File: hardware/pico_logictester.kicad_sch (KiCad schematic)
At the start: 29 parts, among them J1 LOGIC_INPUT, J2 GPIO_5_28, J3 AKKU, J4 STEP_UP_IN, J5 5V VERSORGUNG, J6 TFT Display, Q1 AO3401A, Q2 BC547, SW1 SW_Push, U1 74HC245, U2 74HC245

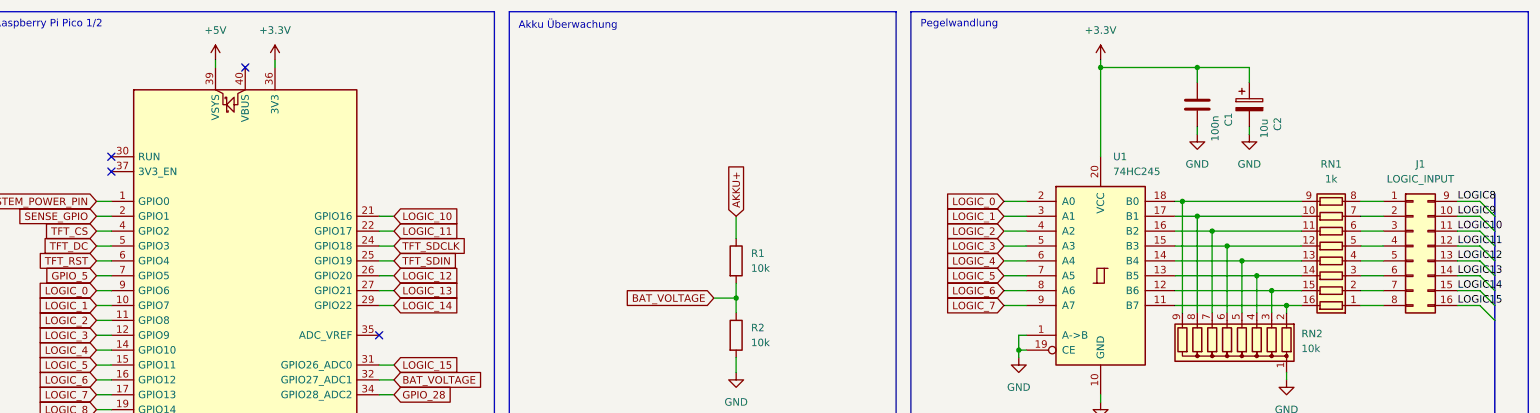
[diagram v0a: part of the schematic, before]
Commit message: Autorouting im Livestream. noch 6 offene Verbindungen!
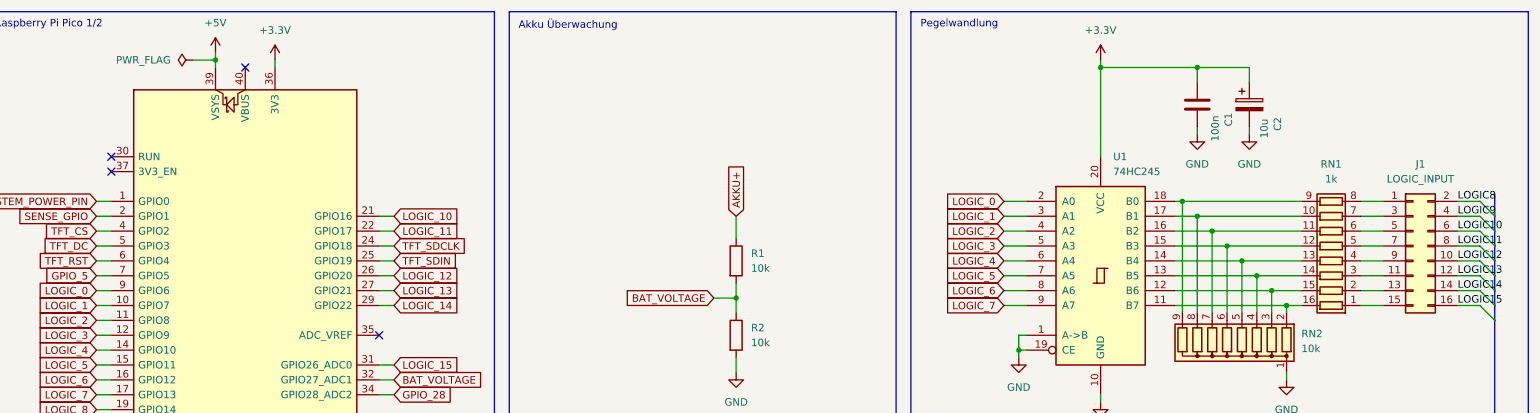
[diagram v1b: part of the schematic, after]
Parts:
- removed J1: LOGIC_INPUT, connector_tk:PinHeader_2x08_P2.54mm_Horizontal_cw, symbol Connector_Generic:Conn_02x08_Top_Bottom
- added J1: LOGIC_INPUT, Connector_IDC:IDC-Header_2x08_P2.54mm_Horizontal, symbol Connector_Generic:Conn_02x08_Odd_Even
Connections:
- net LOGIC10: now also J1.6 (Pin_6)
- net LOGIC11: now also J1.8 (Pin_8)
- net LOGIC12: now also J1.10 (Pin_10)
- net LOGIC13: now also J1.12 (Pin_12)
- net LOGIC14: now also J1.14 (Pin_14)
- net LOGIC15: now also J1.16 (Pin_16)
- net LOGIC8: now also J1.2 (Pin_2)
- net LOGIC9: now also J1.4 (Pin_4)
- net at RN1.8 (R8.1): now also J1.1 (Pin_1)
- net at RN1.7 (R7.1): now also J1.3 (Pin_3)
- net at RN1.6 (R6.1): now also J1.5 (Pin_5)
- net at RN1.5 (R5.1): now also J1.7 (Pin_7)
- net at RN1.4 (R4.1): now also J1.9 (Pin_9)
- net at RN1.3 (R3.1): now also J1.11 (Pin_11)
- net at RN1.2 (R2.1): now also J1.13 (Pin_13)
- net at RN1.1 (R1.1): now also J1.15 (Pin_15)
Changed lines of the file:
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@@
 	)
 	(junction
+		(at 58.42 22.86)
+		(diameter 0)
+		(color 0 0 0 0)
+	)
+	(junction
 		(at 226.06 99.06)
 		(diameter 0)
@@
 	(wire
 		(pts
-			(xy 58.42 22.86) (xy 58.42 24.13)
+			(xy 58.42 21.59) (xy 58.42 22.86)
 		)
 		(stroke
@@
 	(wire
 		(pts
+			(xy 58.42 22.86) (xy 58.42 24.13)
+		)
+		(stroke
+			(width 0)
+			(type default)
+		)
+	)
+	(wire
+		(pts
 			(xy 86.36 52.07) (xy 88.9 52.07)
 		)
@@
 	(wire
 		(pts
+			(xy 54.61 22.86) (xy 58.42 22.86)
+		)
+		(stroke
+			(width 0)
+			(type default)
+		)
+	)
+	(wire
+		(pts
 			(xy 195.58 72.39) (xy 195.58 73.66)
 		)
@@
 	)
 	(symbol
-		(lib_id "Connector_Generic:Conn_02x08_Top_Bottom")
-		(at 262.89 54.61 0)
-		(unit 1)
-		(exclude_from_sim no)
-		(in_bom yes)
-		(on_board yes)
-		(dnp no)
-		(fields_autoplaced yes)
-		(property "Reference" "J1"
-			(at 264.16 40.64 0)
-			(effects
-				(font
-					(size 1.27 1.27)
-				)
-			)
-		)
-		(property "Value" "LOGIC_INPUT"
-			(at 264.16 43.18 0)
-			(effects
-				(font
-					(size 1.27 1.27)
-				)
-			)
-		)
-		(property "Footprint" "connector_tk:PinHeader_2x08_P2.54mm_Horizontal_cw"
-			(at 262.89 54.61 0)
-			(effects
-				(font
-					(size 1.27 1.27)
-				)
-				(hide yes)
-			)
-		)
-		(property "Datasheet" "~"
-			(at 262.89 54.61 0)
-			(effects
-				(font
-					(size 1.27 1.27)
-				)
-				(hide yes)
-			)
-		)
-		(property "Description" "Generic connector, double row, 02x08, top/bottom pin numbering scheme (row 1: 1...pins_per_row, row2: pins_per_row+1 ... num_pins), script generated (kicad-library-utils/schlib/autogen/connector/)"
-			(at 262.89 54.61 0)
-			(effects
-				(font
-					(size 1.27 1.27)
-				)
-				(hide yes)
-			)
-		)
-		(pin "6"
-		)
-		(pin "10"
-		)
-		(pin "16"
-		)
-		(pin "13"
-		)
-		(pin "3"
-		)
-		(pin "2"
-		)
-		(pin "11"
-		)
-		(pin "4"
-		)
-		(pin "7"
-		)
-		(pin "12"
-		)
-		(pin "9"
-		)
-		(pin "5"
-		)
-		(pin "8"
-		)
-		(pin "15"
-		)
-		(pin "1"
-		)
-		(pin "14"
-		)
-		(instances
-			(project ""
-				(path "/ab4c5817-8853-4523-896c-e7a16e8d82cb"
-					(reference "J1")
-					(unit 1)
-				)
-			)
-		)
-	)
-	(symbol
 		(lib_id "Connector_Generic:Conn_01x08")
 		(at 46.99 166.37 0)
@@
 	(symbol
 		(lib_id "power:+5V")
-		(at 58.42 22.86 0)
+		(at 58.42 21.59 0)
 		(unit 1)
 		(exclude_from_sim no)
@@
 		(fields_autoplaced yes)
 		(property "Reference" "#PWR03"
-			(at 58.42 26.67 0)
+			(at 58.42 25.4 0)
 			(effects
 				(font
@@
 		)
 		(property "Value" "+5V"
-			(at 58.42 17.78 0)
+			(at 58.42 16.51 0)
 			(effects
 				(font
@@
 		)
 		(property "Footprint" ""
-			(at 58.42 22.86 0)
+			(at 58.42 21.59 0)
 			(effects
 				(font
@@
 		)
 		(property "Datasheet" ""
-			(at 58.42 22.86 0)
+			(at 58.42 21.59 0)
 			(effects
 				(font
@@
 		)
 		(property "Description" "Power symbol creates a global label with name \"+5V\""
-			(at 58.42 22.86 0)
+			(at 58.42 21.59 0)
 			(effects
 				(font
@@
 	)
 	(symbol
+		(lib_id "power:PWR_FLAG")
+		(at 54.61 22.86 90)
+		(unit 1)
+		(exclude_from_sim no)
+		(in_bom yes)
+		(on_board yes)
+		(dnp no)
+		(fields_autoplaced yes)
+		(property "Reference" "#FLG01"
+			(at 52.705 22.86 0)
+			(effects
+				(font
+					(size 1.27 1.27)
+				)
+				(hide yes)
+			)
+		)
+		(property "Value" "PWR_FLAG"
+			(at 50.8 22.8599 90)
+			(effects
+				(font
+					(size 1.27 1.27)
+				)
+				(justify left)
+			)
+		)
+		(property "Footprint" ""
+			(at 54.61 22.86 0)
+			(effects
+				(font
+					(size 1.27 1.27)
+				)
+				(hide yes)
+			)
+		)
+		(property "Datasheet" "~"
+			(at 54.61 22.86 0)
+			(effects
+				(font
+					(size 1.27 1.27)
+				)
+				(hide yes)
+			)
+		)
+		(property "Description" "Special symbol for telling ERC where power comes from"
+			(at 54.61 22.86 0)
+			(effects
+				(font
+					(size 1.27 1.27)
+				)
+				(hide yes)
+			)
+		)
+		(pin "1"
+		)
+		(instances
+			(project ""
+				(path "/ab4c5817-8853-4523-896c-e7a16e8d82cb"
+					(reference "#FLG01")
+					(unit 1)
+				)
+			)
+		)
+	)
+	(symbol
 		(lib_id "power:GND")
 		(at 87.63 86.36 0)
@@
 					(unit 1)
 				)
+			)
+		)
+	)
+	(symbol
+		(lib_id "Connector_Generic:Conn_02x08_Odd_Even")
+		(at 262.89 54.61 0)
+		(unit 1)
+		(exclude_from_sim no)
+		(in_bom yes)
+		(on_board yes)
+		(dnp no)
+		(fields_autoplaced yes)
+		(property "Reference" "J1"
+			(at 264.16 40.64 0)
+			(effects
+				(font
+					(size 1.27 1.27)
+				)
+			)
+		)
+		(property "Value" "LOGIC_INPUT"
+			(at 264.16 43.18 0)
+			(effects
+				(font
+					(size 1.27 1.27)
+				)
+			)
+		)
+		(property "Footprint" "Connector_IDC:IDC-Header_2x08_P2.54mm_Horizontal"
+			(at 262.89 54.61 0)
+			(effects
+				(font
+					(size 1.27 1.27)
+				)
+				(hide yes)
+			)
+		)
+		(property "Datasheet" "~"
+			(at 262.89 54.61 0)
+			(effects
+				(font
+					(size 1.27 1.27)
+				)
+				(hide yes)
+			)
+		)
+		(property "Description" "Generic connector, double row, 02x08, odd/even pin numbering scheme (row 1 odd numbers, row 2 even numbers), script generated (kicad-library-utils/schlib/autogen/connector/)"
+			(at 262.89 54.61 0)
+			(effects
+				(font
+					(size 1.27 1.27)
+				)
+				(hide yes)
+			)
+		)
+		(pin "4"
+		)
+		(pin "12"
+		)
+		(pin "6"
+		)
+		(pin "2"
+		)
+		(pin "11"
+		)
+		(pin "13"
+		)
+		(pin "7"
+		)
+		(pin "1"
+		)
+		(pin "9"
+		)
+		(pin "14"
+		)
+		(pin "8"
+		)
+		(pin "16"
+		)
+		(pin "10"
+		)
+		(pin "15"
+		)
+		(pin "5"
+		)
+		(pin "3"
+		)
+		(instances
+			(project ""
+				(path "/ab4c5817-8853-4523-896c-e7a16e8d82cb"
+					(reference "J1")
+					(unit 1)
+				)
